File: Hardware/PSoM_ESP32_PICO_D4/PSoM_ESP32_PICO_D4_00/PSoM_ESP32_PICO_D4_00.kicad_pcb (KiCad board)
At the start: 6 copper layers, 26.3 x 23.2 mm, 58 parts, among them J101 DF40C-60DP-0.4V(51), J102 Bare PCB USB C, SW401 SW_Push, SW402 SW_Push, U201 BQ24075RGTR, U301 MIC5528-3.3YMT-T5, U401 ESP32-S2FH4, Y601 Crystal_GND24_Small

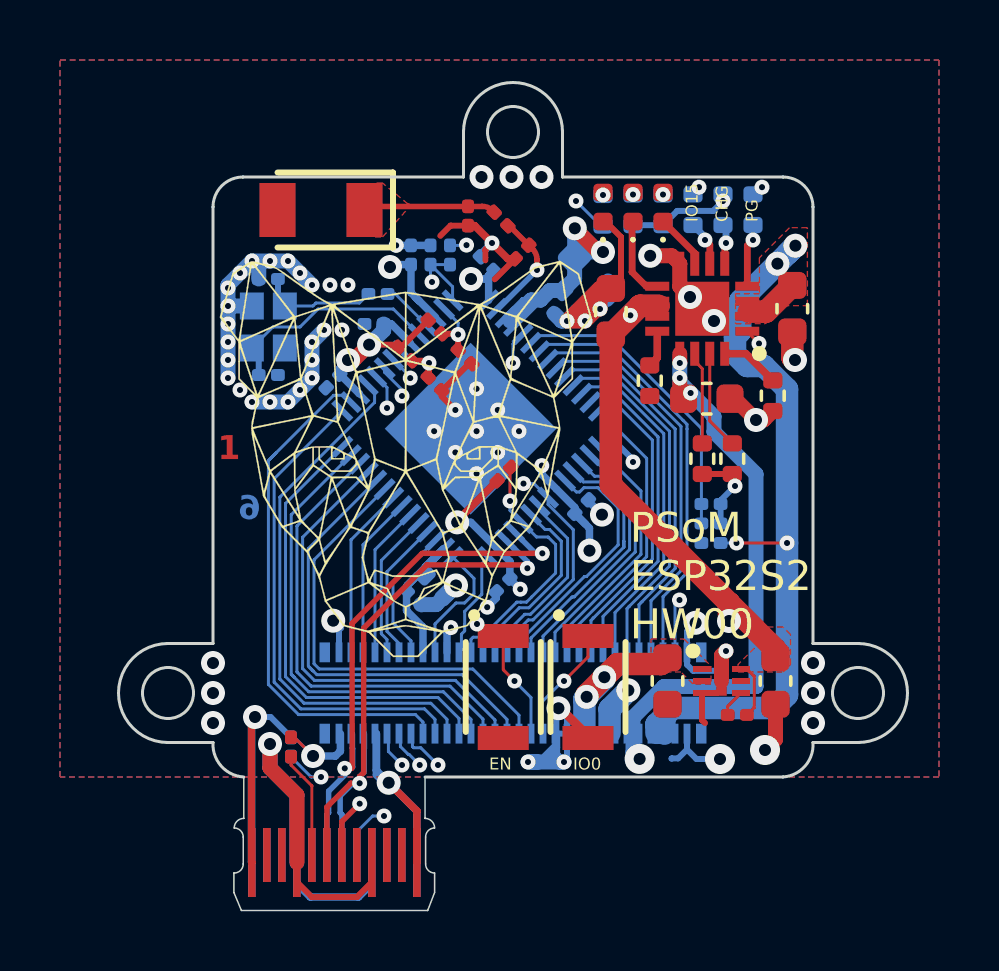
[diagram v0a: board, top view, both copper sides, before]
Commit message: First route for the PICO_D4
Added .gitignore
Modify at your own taste, this one will be tricky
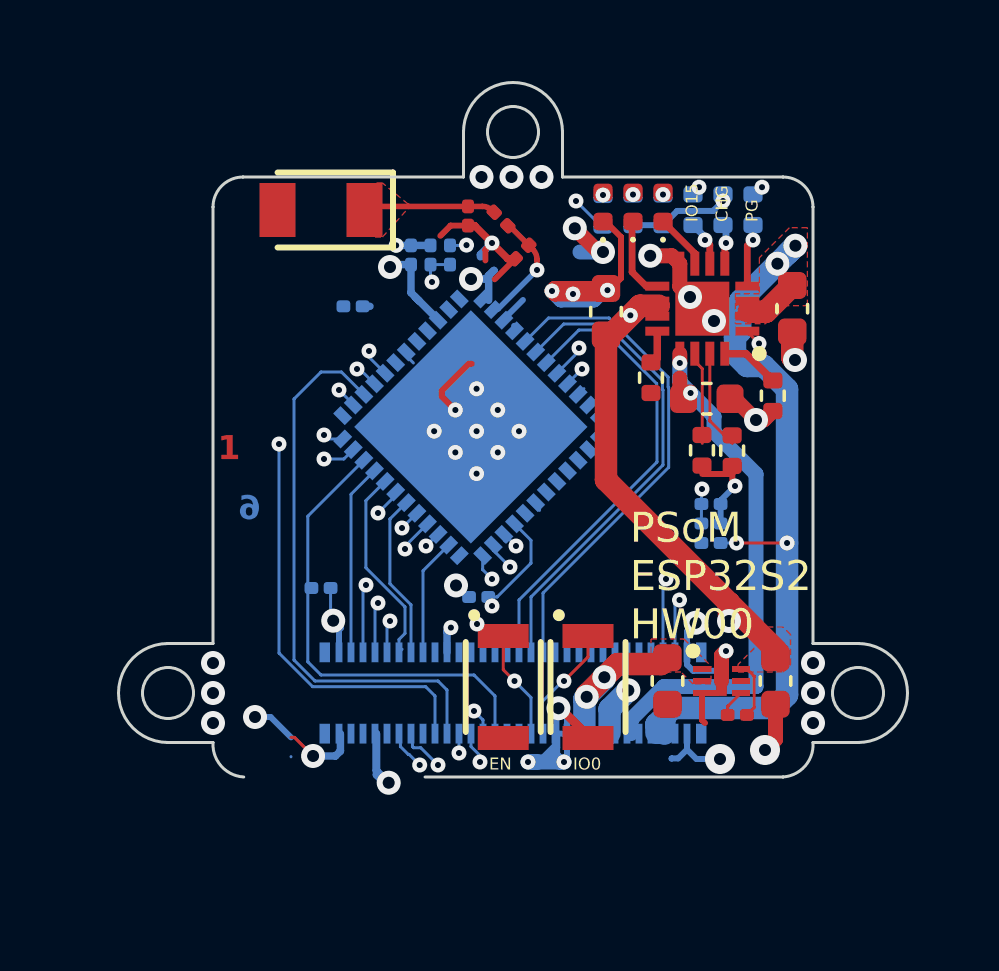
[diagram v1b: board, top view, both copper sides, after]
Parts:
- removed the C401 at (127.8, 92.4)
- removed the C402 at (127.8, 95.6)
- removed the C403 at (130.0, 95.8)
- removed C408, C411, C412, C415, C416: 100n, Capacitor_SMD:C_0201_0603Metric
- removed C409: 10u, Capacitor_SMD:C_0603_1608Metric
- removed C410, C413: 1u, Capacitor_SMD:C_0402_1005Metric
- removed G***: LOGO, Component_lib:puma_logo_14mm
- removed J102: Bare PCB USB C, Component_lib:usb-c-pcb
- removed R101, R102: 5.1k, Resistor_SMD:R_0201_0603Metric
- removed the R401 at (131.5, 92.9)
- removed R404: 10k, Resistor_SMD:R_0201_0603Metric
- removed R405, R406, R407: nu, Resistor_SMD:R_0201_0603Metric
- removed Y601: Crystal_GND24_Small, Component_lib:Crystal_SMD_2016-4Pin_2.0x1.6mm
- added R409: nu, Resistor_SMD:R_0201_0603Metric, B.Cu at (129.6, 102.7)
- C401: renamed from C404; value 100n -> 10u
- R408: moved to B.Cu
- U401: value ESP32-S2FH4 -> ESP32-PICO-D4; footprint Component_lib:QFN40P700X700X90-57N-D -> Components_NdG:ESP32-PICO-D4_1
- moved R408 7.25 mm to (134.9, 103.0), turned to 180 degrees
- moved C402 0.92 mm to (130.7, 93.3)
- moved R202 0.28 mm to (142.3, 98.1)
- moved R201 0.27 mm to (143.3, 98.1)
- moved C203 0.16 mm to (139.1, 93.5)
- moved R204 0.11 mm to (140.6, 95.7)
- renumbered C405 to C402, C406 to C403, C407 to C404, C414 to C405, R402 to R401, R403 to R402, SW402 to SW401, SW401 to SW402
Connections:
- net /400_ESP32/LNA_IN renamed /400_ESP32/LAN_IN
- C101 pad 1: IO1 -> IO39
- J101 pad 11: IO5 -> IO18
- J101 pad 13: IO6 -> IO19
- J101 pad 15: IO7 -> IO21
- J101 pad 17: IO8 -> IO34
- J101 pad 19: IO9 -> IO32
- J101 pad 21: IO10 -> IO33
- J101 pad 23: IO11 -> IO35
- J101 pad 25: IO12 -> IO36
- J101 pad 27: IO13 -> IO37
- J101 pad 29: IO14 -> IO38
- J101 pad 30: IO33 -> unconnected-(J101-Pad30)
- J101 pad 31: IO15 -> unconnected-(J101-Pad31)
- J101 pad 32: IO34 -> unconnected-(J101-Pad32)
- J101 pad 33: IO16 -> unconnected-(J101-Pad33)
- J101 pad 34: IO35 -> IO5
- J101 pad 35: IO17 -> IO25
- J101 pad 36: IO36 -> IO15
- J101 pad 37: IO18 -> IO26
- J101 pad 38: IO37 -> IO12
- J101 pad 39: IO21 -> unconnected-(J101-Pad39)
- J101 pad 40: IO38 -> IO9
- J101 pad 42: IO41 -> IO22
- J101 pad 43: SPI7 -> unconnected-(J101-Pad43)
- J101 pad 44: IO39 -> IO23
- J101 pad 46: IO40 -> IO27
- J101 pad 5: IO2 -> IO4
- J101 pad 52: IO42 -> unconnected-(J101-Pad52)
- J101 pad 56: /100_Connectors/D+ -> unconnected-(J101-Pad56)
- J101 pad 58: /100_Connectors/D- -> unconnected-(J101-Pad58)
- J101 pad 7: IO3 -> IO13
- J101 pad 9: IO4 -> IO14
- R103 pad 2: IO1 -> IO39
- R104 pad 1: IO1 -> IO39
- R401 pad 1: IO15 -> IO2
- R408 pad 1: /400_ESP32/IO45 -> IO15
- U401 pad 10: IO5 -> IO34
- U401 pad 11: IO6 -> IO35
- U401 pad 12: IO7 -> IO32
- U401 pad 13: IO8 -> IO33
- U401 pad 14: IO9 -> IO25
- U401 pad 15: IO10 -> IO26
- U401 pad 16: IO11 -> IO27
- U401 pad 17: IO12 -> IO14
- U401 pad 18: IO13 -> IO12
- U401 pad 19: IO14 -> +3V3
- U401 pad 20: +3V3 -> IO13
- U401 pad 22: IO16 -> IO2
- U401 pad 23: IO17 -> IO0
- U401 pad 24: IO18 -> IO4
- U401 pad 25: /100_Connectors/D- -> unconnected-(U401-GPIO16-Pad25)
- U401 pad 26: /100_Connectors/D+ -> SPI6
- U401 pad 27: +3V3 -> SPI1
- U401 pad 28: IO21 -> IO9
- U401 pad 29: SPI7 -> SPI3
- U401 pad 30: SPI6 -> SPI5
- U401 pad 31: SPI5 -> SPI2
- U401 pad 33: SPI3 -> SPI0
- U401 pad 34: SPI2 -> IO5
- U401 pad 35: SPI1 -> IO18
- U401 pad 36: SPI0 -> IO23
- U401 pad 37: IO33 -> +3V3
- U401 pad 38: IO34 -> IO19
- U401 pad 39: IO35 -> IO22
- U401 pad 40: IO36 -> /100_Connectors/TX0
- U401 pad 41: IO37 -> /100_Connectors/RX0
- U401 pad 42: IO38 -> IO21
- U401 pad 43: IO39 -> +3V3
- U401 pad 44: IO40 -> unconnected-(U401-NC-Pad44)
- U401 pad 45: +3V3 -> unconnected-(U401-NC-Pad45)
- U401 pad 46: IO41 -> +3V3
- U401 pad 47: IO42 -> unconnected-(U401-CAP2-Pad47)
- U401 pad 48: /100_Connectors/TX0 -> unconnected-(U401-CAP1-Pad48)
- U401 pad 49: /100_Connectors/RX0 -> GND
- U401 pad 5: IO0 -> IO36
- U401 pad 6: IO1 -> IO37
- U401 pad 7: IO2 -> IO38
- U401 pad 8: IO3 -> IO39
- U401 pad 9: IO4 -> /100_Connectors/EN
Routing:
- net GND: track 96.0 -> 62.6 mm, vias 71 -> 44
- net VBUS: track 48.9 -> 17.8 mm, vias 5 -> 2
- net +3V3: track 36.4 -> 14.8 mm, vias 13 -> 7
- net /100_Connectors/D-: track 21.5 -> 0.00 mm, vias 3 -> 0
- net /100_Connectors/D+: track 20.4 -> 0.00 mm, vias 2 -> 0
- net IO22: track 0.00 -> 18.7 mm
- net IO41: track 17.8 -> 0.00 mm
- net IO40: track 17.6 -> 0.00 mm
- net IO23: track 0.00 -> 16.3 mm, vias 0 -> 2
- net IO42: track 15.3 -> 0.00 mm, vias 2 -> 0
- net IO35: track 15.0 -> 0.00 mm
- net IO33: track 15.0 -> 0.00 mm
- net IO34: track 15.1 -> 0.28 mm
- net IO3: track 13.5 -> 0.00 mm
- net IO6: track 11.8 -> 0.00 mm
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- removed copper zone on In2.Cu, net +3V3
- removed copper zone on B.Cu, net GND
- removed copper zone on F.Cu, net GND
- removed copper zone on In4.Cu, net GND
